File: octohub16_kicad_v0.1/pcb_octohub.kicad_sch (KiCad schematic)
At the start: 9 parts, among them J101 USB_C_Receptacle_USB2.0, U101 AMS1117-3.3

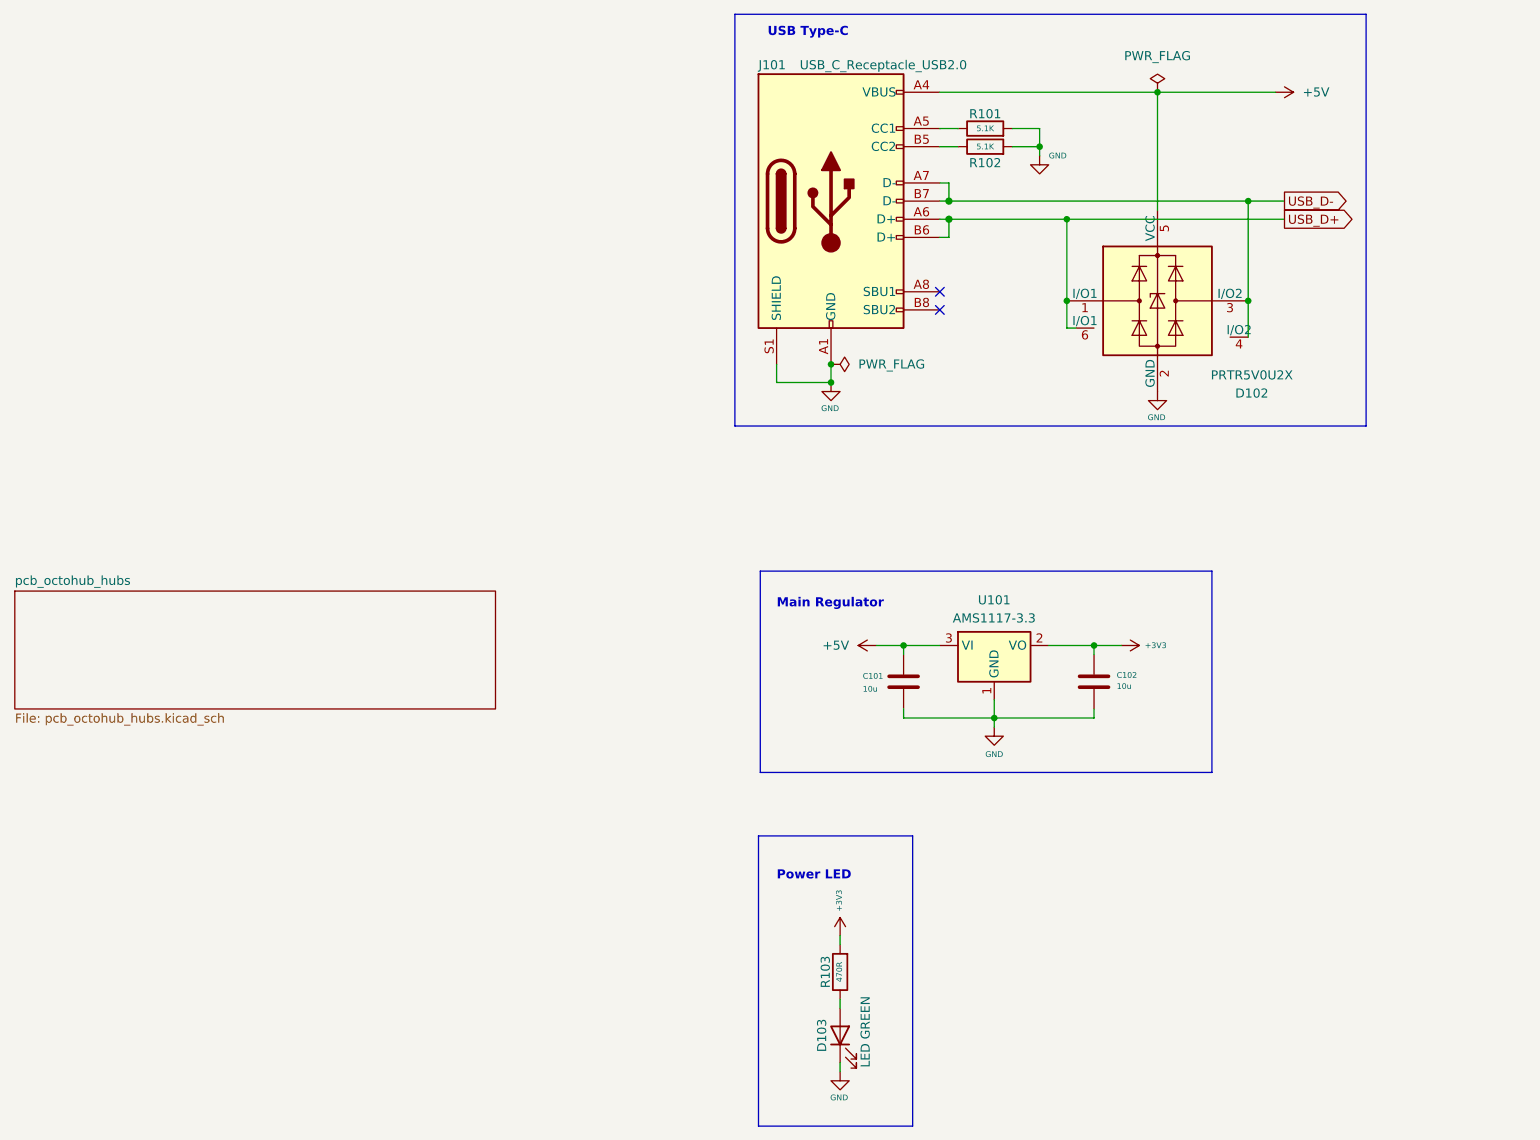
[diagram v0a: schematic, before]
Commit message: experiment octohub16
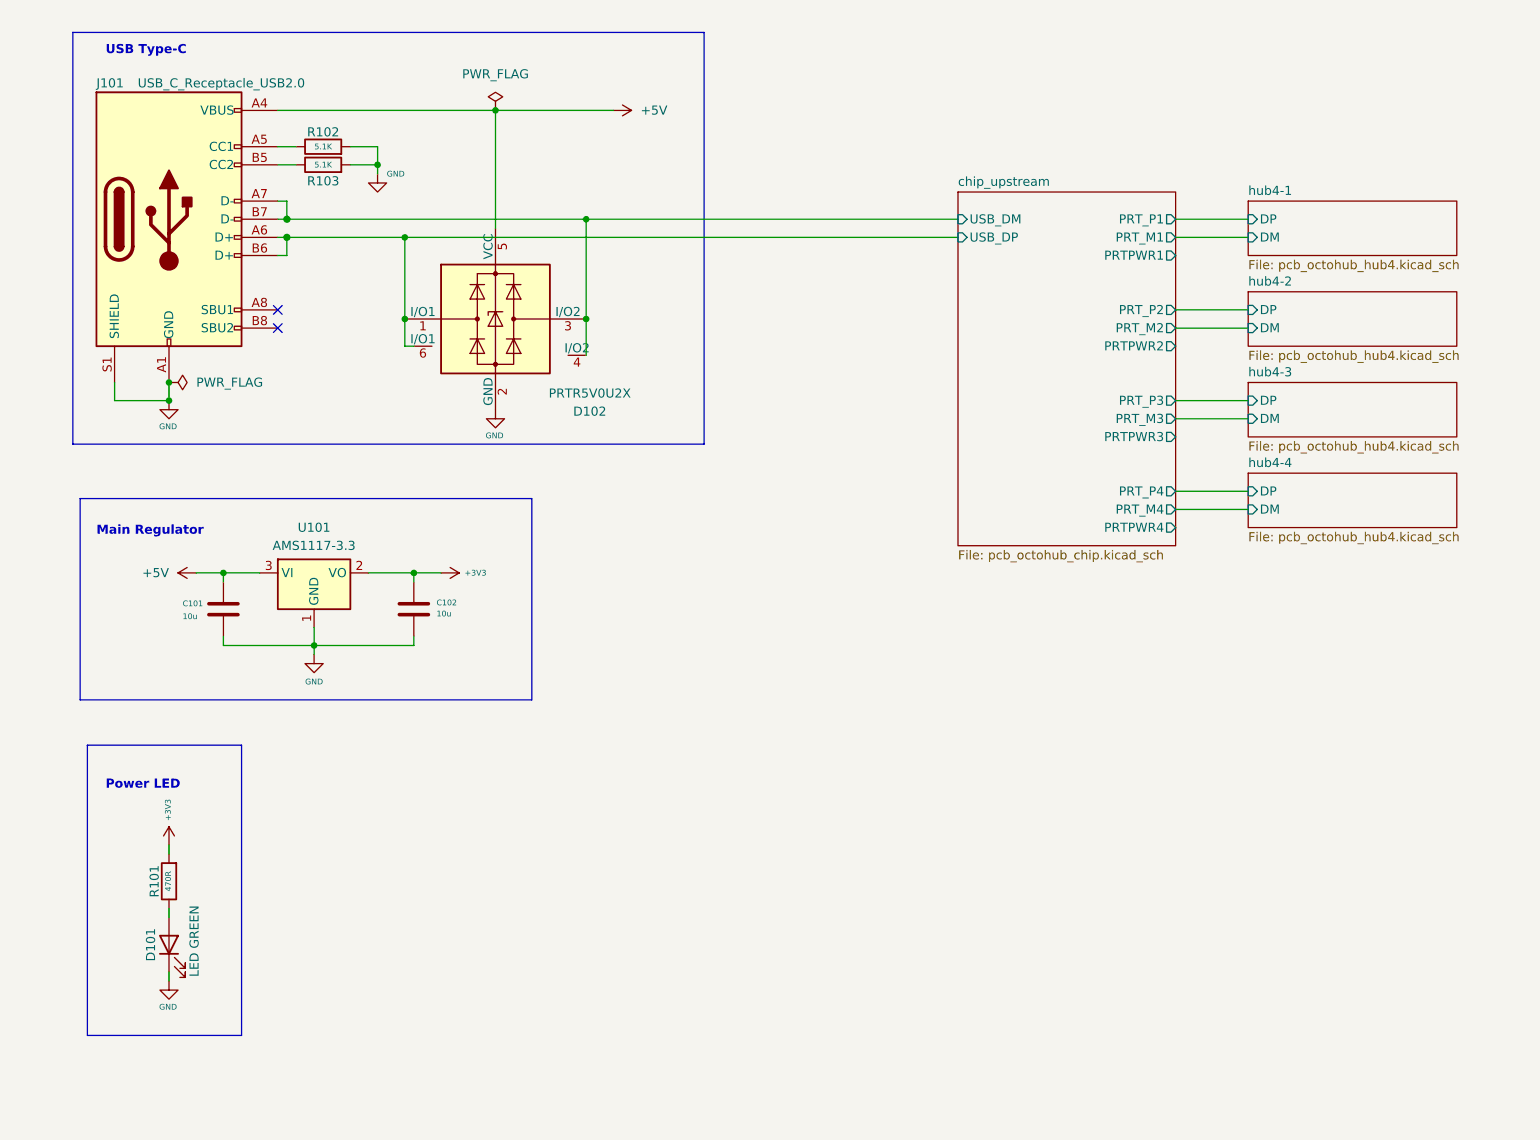
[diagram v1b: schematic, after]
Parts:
- renumbered D103 to D101, R103 to R101, R101 to R102, R102 to R103
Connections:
- net USB_D+ renamed chip_upstream/USB_DP
- net USB_D- renamed chip_upstream/USB_DM
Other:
- removed sheet pcb_octohub_hubs
- added sheet chip_upstream (pcb_octohub_chip.kicad_sch)
- added sheet hub4-1 (pcb_octohub_hub4.kicad_sch)
- added sheet hub4-2 (pcb_octohub_hub4.kicad_sch)
- added sheet hub4-3 (pcb_octohub_hub4.kicad_sch)
- added sheet hub4-4 (pcb_octohub_hub4.kicad_sch)
- moved on the sheet: C101, C102, D101, D102, J101, R101, R102, R103, U101
